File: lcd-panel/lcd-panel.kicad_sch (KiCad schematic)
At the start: 46 parts, among them J1 USB wire, J2 LCD FPC connector, J3 Fan Socket, J4 TC2030, Q1 AO3400A, Q2 AO3401A, Q3 AO3400A, U1 FT232HL-REEL, U2 93LC56BT-I/OT, U3 USBLC6-2SC6, U4 ATtiny414-SS, Y1 12 MHz, 20 pF load

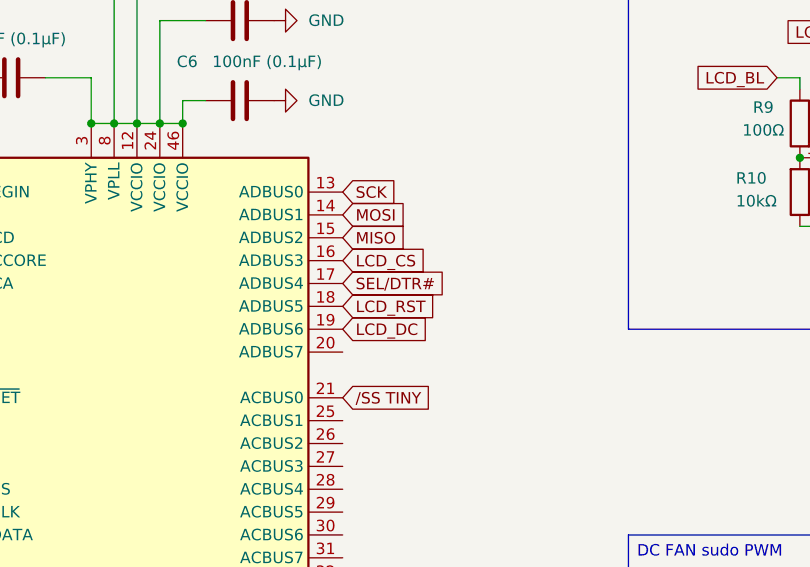
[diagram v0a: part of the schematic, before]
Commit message: Wiring most of the components together
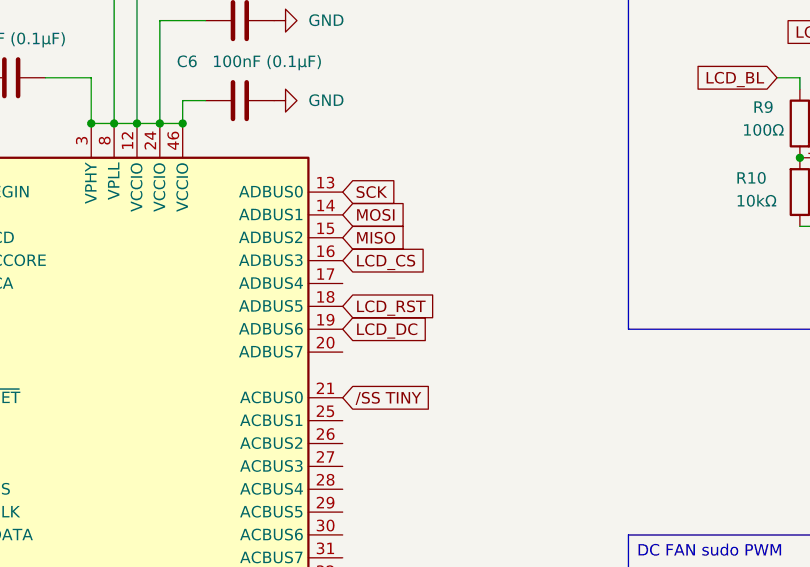
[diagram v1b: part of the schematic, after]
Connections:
- net SEL/DTR#: no longer names the net of U1.17 (ADBUS4)
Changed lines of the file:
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@@
-		)
-	)
-	(global_label "SEL{slash}DTR#"
-		(shape input)
-		(at 184.15 66.04 0)
-		(fields_autoplaced yes)
-		(effects
-			(font
-				(size 1.27 1.27)
-			)
-			(justify left)
-		)
-		(property "Intersheetrefs" "${INTERSHEET_REFS}"
-			(at 196.6299 66.04 0)
-			(effects
-				(font
-					(size 1.27 1.27)
-				)
-				(justify left)
-				(hide yes)
-			)
 		)
 	)
